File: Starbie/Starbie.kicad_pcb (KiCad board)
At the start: 2 copper layers, 132.5 x 127.5 mm, 11 parts, among them J1 Conn_01x04_Pin, J2 Conn_01x08_Pin, J3 USB_C_Receptacle_USB2.0_14P, SW1 SW_Push, SW2 SW_Push, U1 XIAO-ESP32-C3-SMD, U2 DHT11

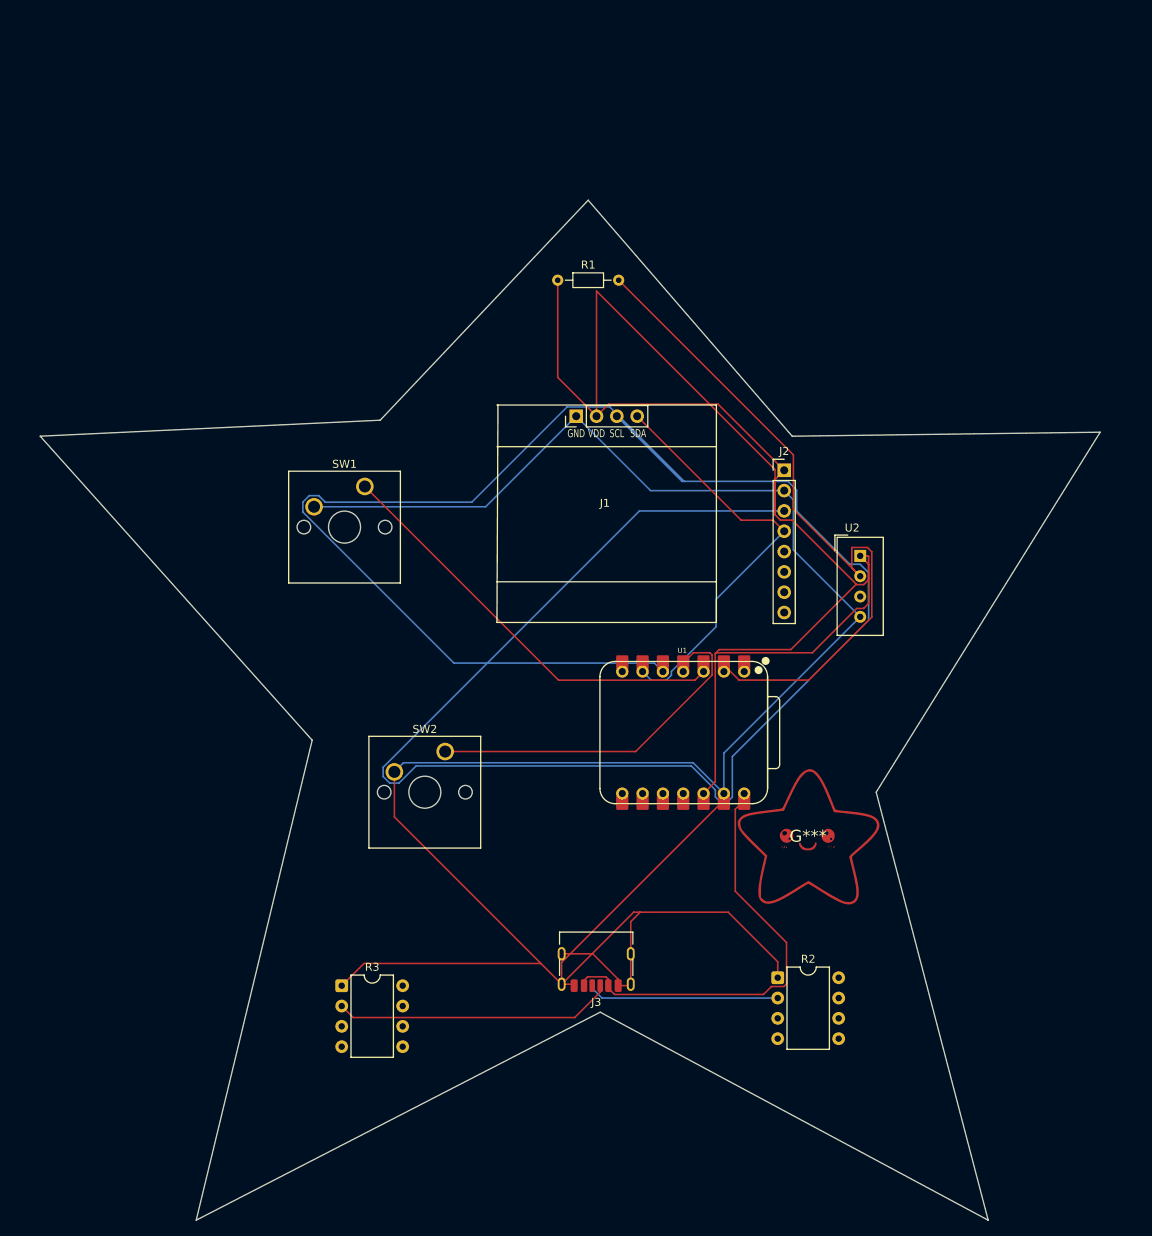
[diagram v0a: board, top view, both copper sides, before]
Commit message: added more and changed shape
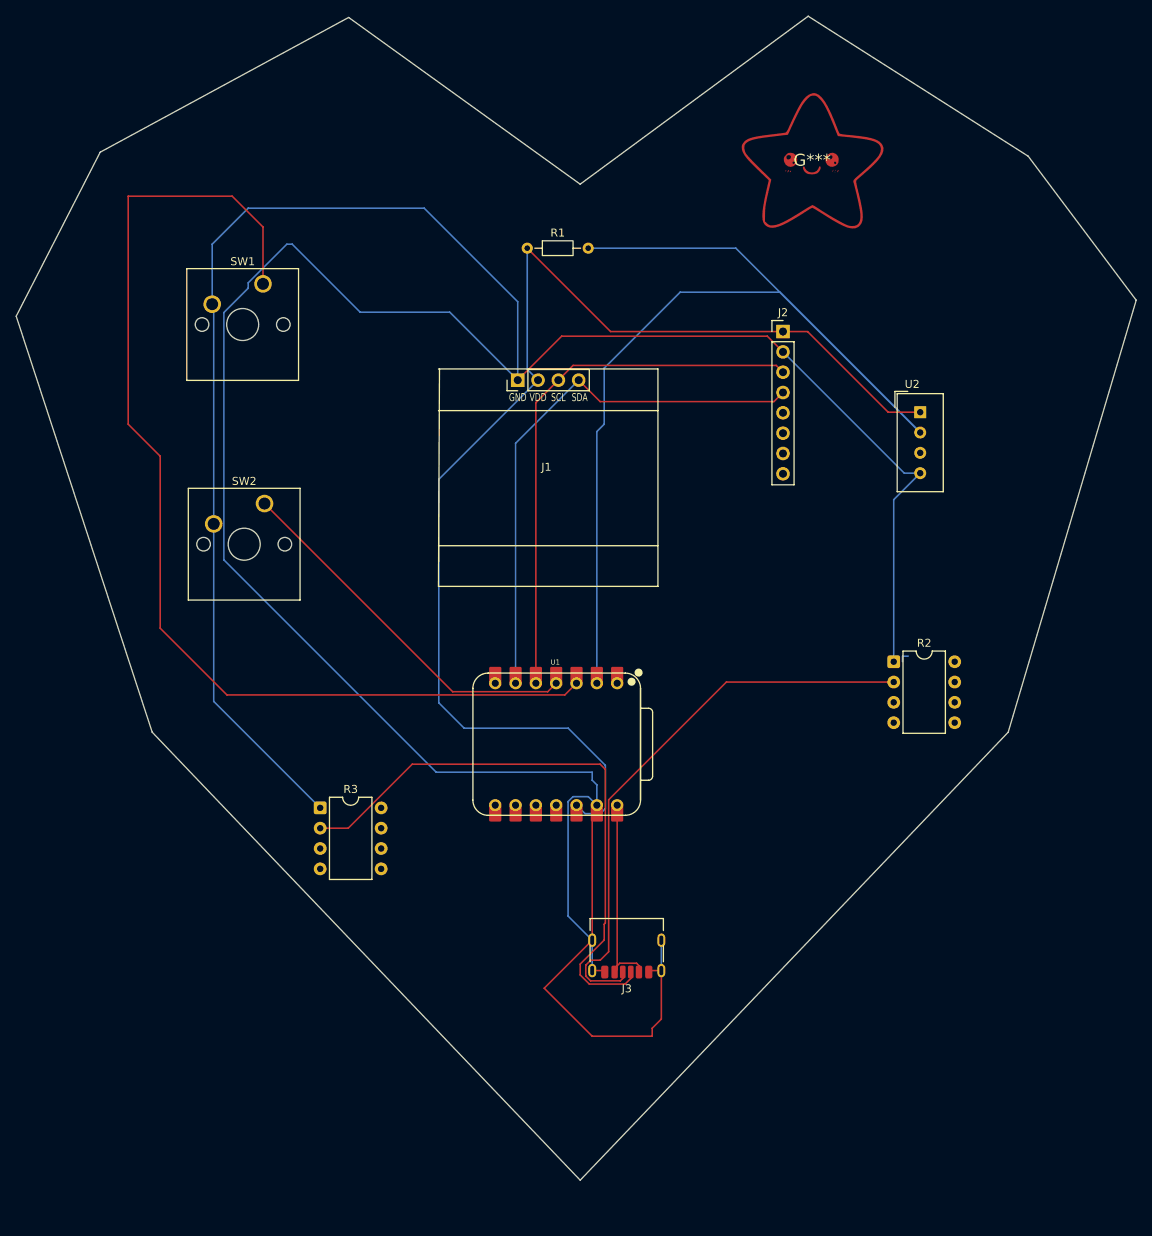
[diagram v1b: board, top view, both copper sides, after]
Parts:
- moved G*** 84.5 mm to (146.0, 57.0)
- moved R2 42.1 mm to (156.2, 119.7)
- moved SW2 38.4 mm to (77.5, 99.9)
- moved SW1 28.3 mm to (77.3, 72.5)
- moved R3 22.4 mm to (84.5, 138.0)
- moved U2 19.5 mm to (159.5, 88.5)
- moved J2 17.3 mm to (142.3, 78.4)
- moved U1 15.9 mm to (114.0, 130.0)
- moved J1 8.59 mm to (113.0, 84.5)
- moved R1 5.52 mm to (110.4, 68.0)
- moved J3 4.18 mm to (122.8, 155.3)
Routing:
- net /SCL: track 300.1 -> 68.2 mm
- net GND: track 309.3 -> 438.6 mm
- net /GPI02: track 52.8 -> 137.3 mm
- net /DHT11 DATA: track 87.0 -> 141.5 mm
- net /groundi: track 24.0 -> 71.4 mm
- net /ng: track 35.0 -> 74.1 mm
- net +3.3V: track 192.5 -> 153.9 mm
- net +5V: track 54.3 -> 25.7 mm
- net /SDA: track 52.5 -> 68.3 mm
- net /GPIO3: track 45.2 -> 46.8 mm
- net (no net): track 0.00 -> 1.40 mm
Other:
- board size 132.5 x 127.5 mm -> 140 x 145.5 mm
